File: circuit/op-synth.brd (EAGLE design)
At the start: 76.2 x 76.2 mm, 76 parts, among them SW1 OS102011MA1QOS102011MA1Q_TOP

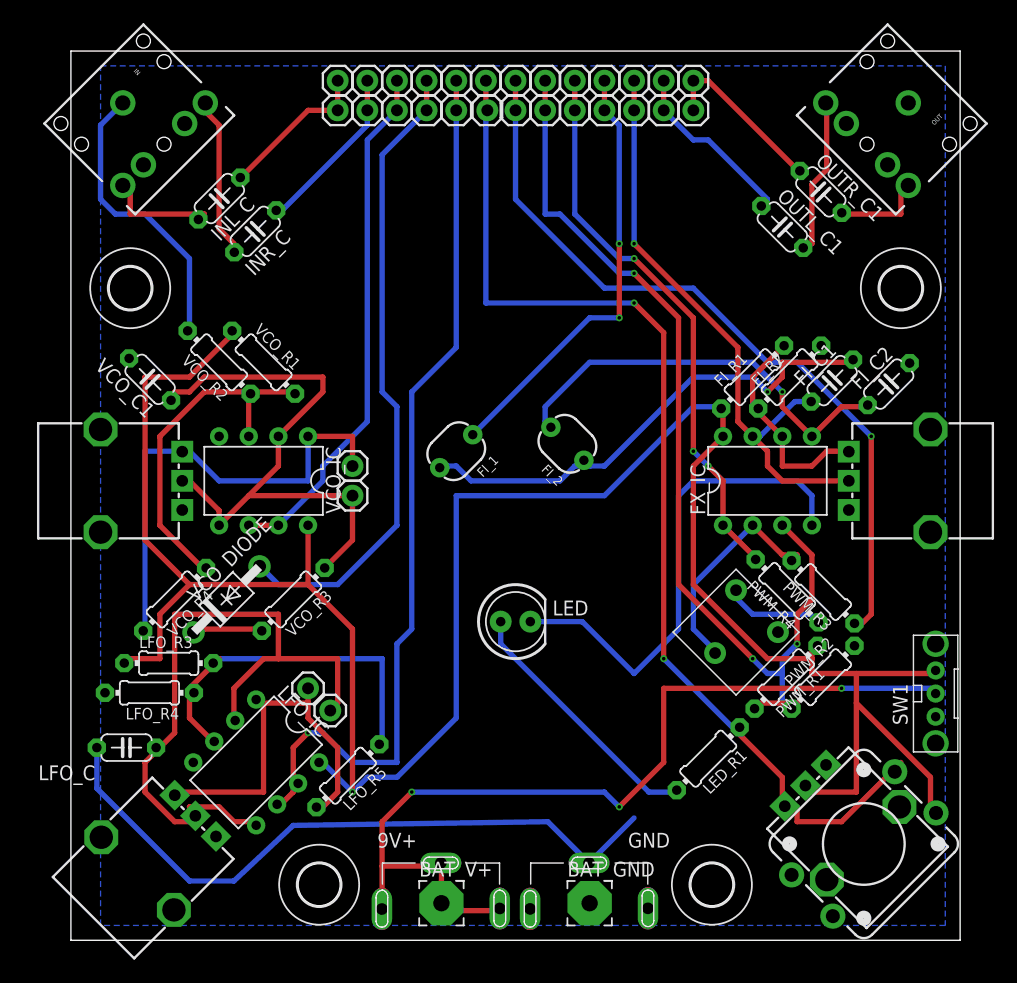
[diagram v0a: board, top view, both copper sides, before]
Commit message: Updated to latest version
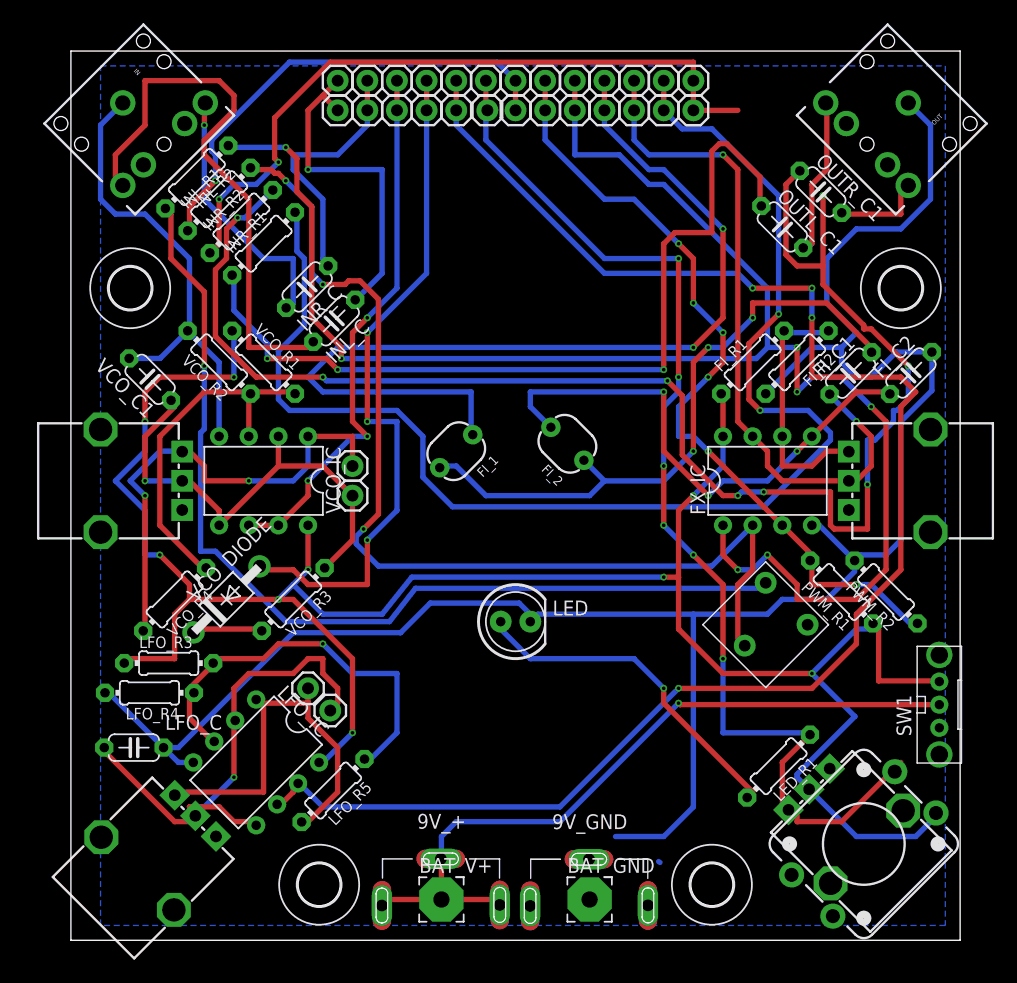
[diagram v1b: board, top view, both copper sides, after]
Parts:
- removed 9V+: KEYSTONE-629+, kanflo:KEYSTONE_BATTAERY_TERMINAL-629+
- removed GND: KEYSTONE-629, kanflo:KEYSTONE_AA_AAA_BATTERY_TERMINAL-629
- removed PWM_R3, PWM_R4: 10k, resistor:0204/7
- added 9V_+: KEYSTONE-637, kanflo:KEYSTONE_AA_AAA_BATTERY_TERMINAL-637
- added 9V_GND: KEYSTONE-629, kanflo:KEYSTONE_AA_AAA_BATTERY_TERMINAL-629
- added INL_R1, INL_R2: 100k, resistor:0204/7
- added INR_R1, INR_R2: 10k, resistor:0204/7
- LED_R1: value 330 -> 150
- PWM_IN, PWM_OUT: value AMP -> PWM
- VCO: value OSC -> VCO
- VCO~: value OSC~ -> VCO~
- ~PWM: value AMP~ -> PWM~
- moved INL_C 14.4 mm to (22.6, 53.1)
- moved PWM_R2 9.08 mm to (69.8, 29.8), turned to 135 degrees
- moved PWM_R1 8.72 mm to (66.0, 29.8), turned to 135 degrees
- moved INR_C 6.51 mm to (20.2, 56.0)
- moved LED_R1 6.07 mm to (60.6, 14.9)
- moved ATTENUATION 2.62 mm to (61.3, 28.8)
- moved FI_C2 2.13 mm to (72.0, 48.6)
- moved LFO_R5 1.80 mm to (22.5, 12.8)
- moved FI_C1 1.71 mm to (66.8, 48.6)
- moved FI_R2 1.42 mm to (62.2, 49.5), turned to 225 degrees
- moved FI_R1 1.27 mm to (58.4, 49.5)
- moved SW1 1.00 mm to (74.4, 20.2)
- moved LFO_C 0.63 mm to (5.40, 16.5), turned to 0 degrees
- moved P_LED 0.45 mm to (68.2, 7.99)
- moved BAT_GND 0.32 mm to (44.5, 3.49)
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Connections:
- removed net MOD_IN: PWM_IN.1, PWM_IN1.1, PWM_R3.1
- removed net N$5 (its old number): ATTENUATION.3, PWM_R4.1
- removed net PWM_OUT: FX_IC.1, PWM_OUT.1, PWM_OUT1.1, PWM_R4.2
- new net N$25: ATTENUATION.1, FX_IC.2, INL_R1.2
- new net N$26: FX_IC.1, INL_R2.1, PWM_OUT.1, PWM_OUT1.1
- new net N$27: INR_R2.2, OUTR_C1.1
- new net N$28: INR_R1.2, OUTL.1, OUTL1.1
- new net N$30: INR_R1.1, OUTL_C1.1
- net GND: now also 9V_GND.GND@1, 9V_GND.GND@2, 9V_GND.GND@3; no longer GND.GND@1, GND.GND@2, GND.GND@3
- net N$1: now also 9V_+.VCC@1, 9V_+.VCC@2, 9V_+.VCC@3; no longer 9V+.V+@1, 9V+.V+@2, 9V+.V+@3
- net N$12: now also INL_R1.1, PWM_IN.1, PWM_IN1.1; no longer OUTL.1, OUTL1.1, OUTL_C1.1
- net N$3: now also ATTENUATION.3, INL_R2.2; no longer ATTENUATION.1, FX_IC.2, PWM_R3.2
- net N$9: now also INR_R2.1; no longer OUTR_C1.1
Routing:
- net N$26: track 0.00 -> 144.3 mm, vias 0 -> 7
- net N$27: track 0.00 -> 127.8 mm, vias 0 -> 8
- net N$28: track 0.00 -> 115.5 mm, vias 0 -> 2
- net GND: track 125.4 -> 218.3 mm
- net N$25: track 0.00 -> 88.5 mm, vias 0 -> 3
- net N$30: track 0.00 -> 73.1 mm, vias 0 -> 3
- net MOD_IN: track 66.6 -> 0.00 mm, vias 1 -> 0
- net N$3: track 19.4 -> 83.4 mm, vias 0 -> 1
- net LFO: track 77.5 -> 140.6 mm, vias 1 -> 4
- net PWM_OUT: track 48.2 -> 0.00 mm, vias 3 -> 0
- net N$9: track 14.8 -> 61.1 mm, vias 0 -> 2
- net FILTER_IN: track 37.8 -> 81.4 mm
- net N$20: track 10.2 -> 48.7 mm
- net N$12: track 15.4 -> 40.9 mm, vias 0 -> 1
- net N$19: track 13.3 -> 29.7 mm, vias 0 -> 1
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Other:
- board text added: "2018-06-14"
- board text added: "500k+"
- board text added: "FILTER"
- board text added: "OP- SYNTH"
- board text added: "POT/SWITCH"
- board text added: "PWM"
- board text added: "PWM~+/-"
- board text added: "Power"
- board text added: "VCO"
- board text removed: "+"
- board text removed: "-"
- board text removed: "500k"
- board text removed: "500k OR BUTTON"
- board text removed: "9V+"
- board text removed: "GAIN"
- board text removed: "GND"
- board text removed: "OP-SYNTH 2018-05-09"
- board text removed: "OSC"
- board text removed: "POWER"
- board text removed: "Q"
